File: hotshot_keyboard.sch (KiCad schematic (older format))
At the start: 25 parts, among them SW1 SW_Push, U1 ATmega32U4-AU, Y1 Crystal_GND24_Small

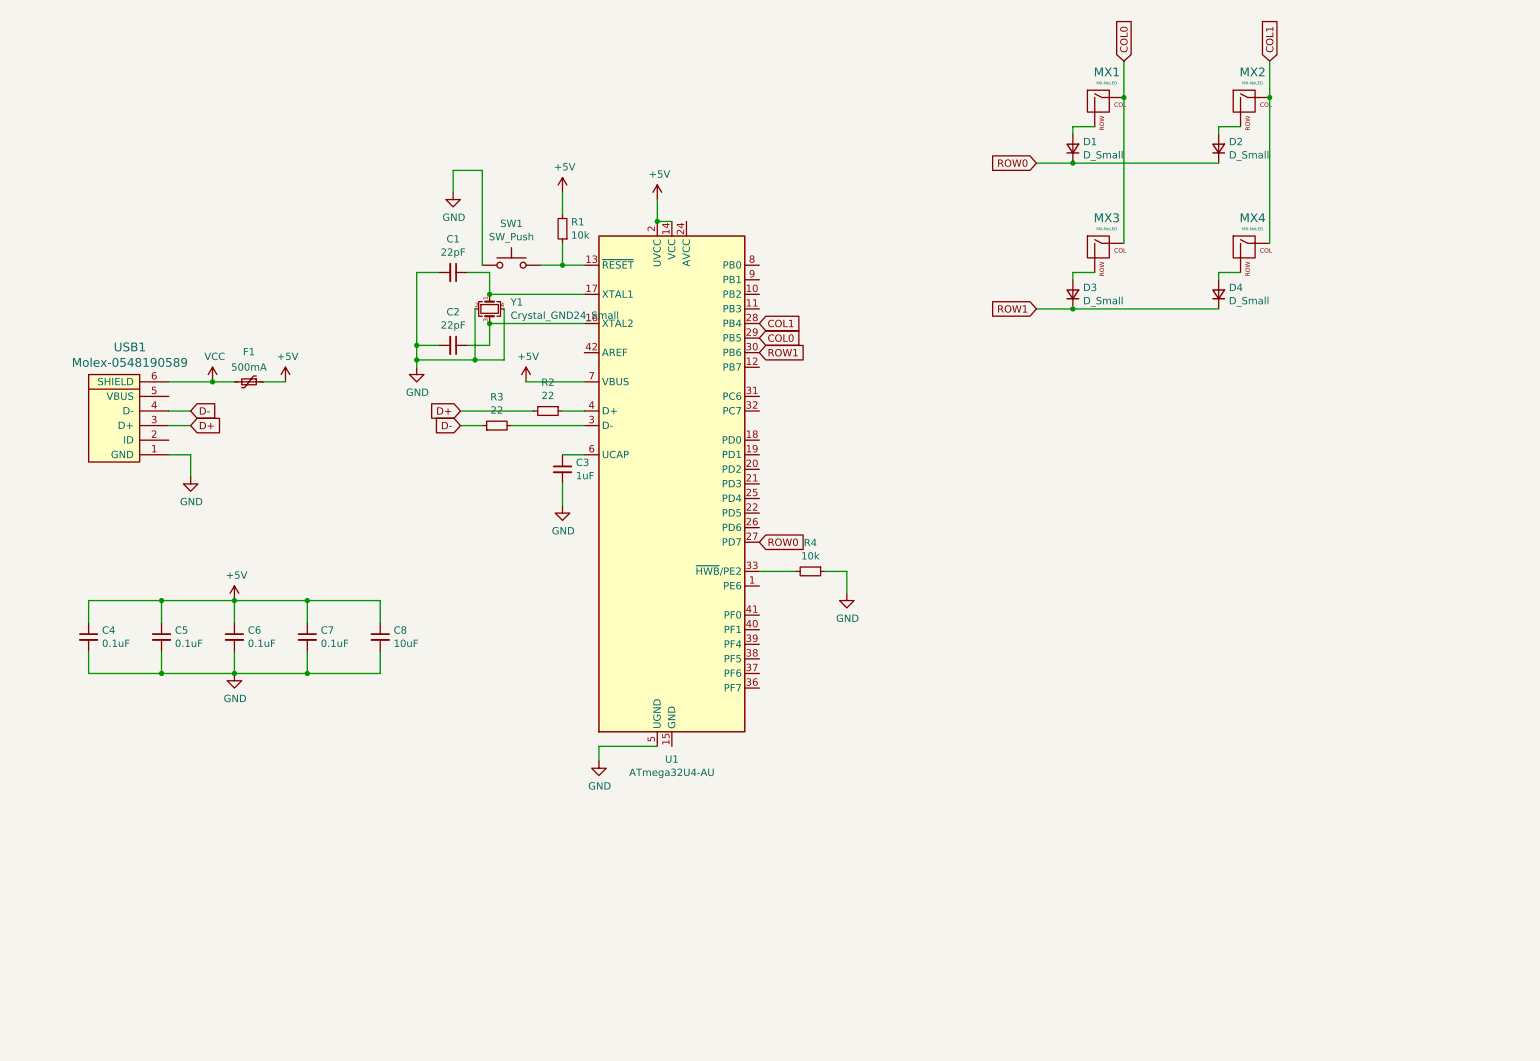
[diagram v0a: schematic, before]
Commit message: update schematics
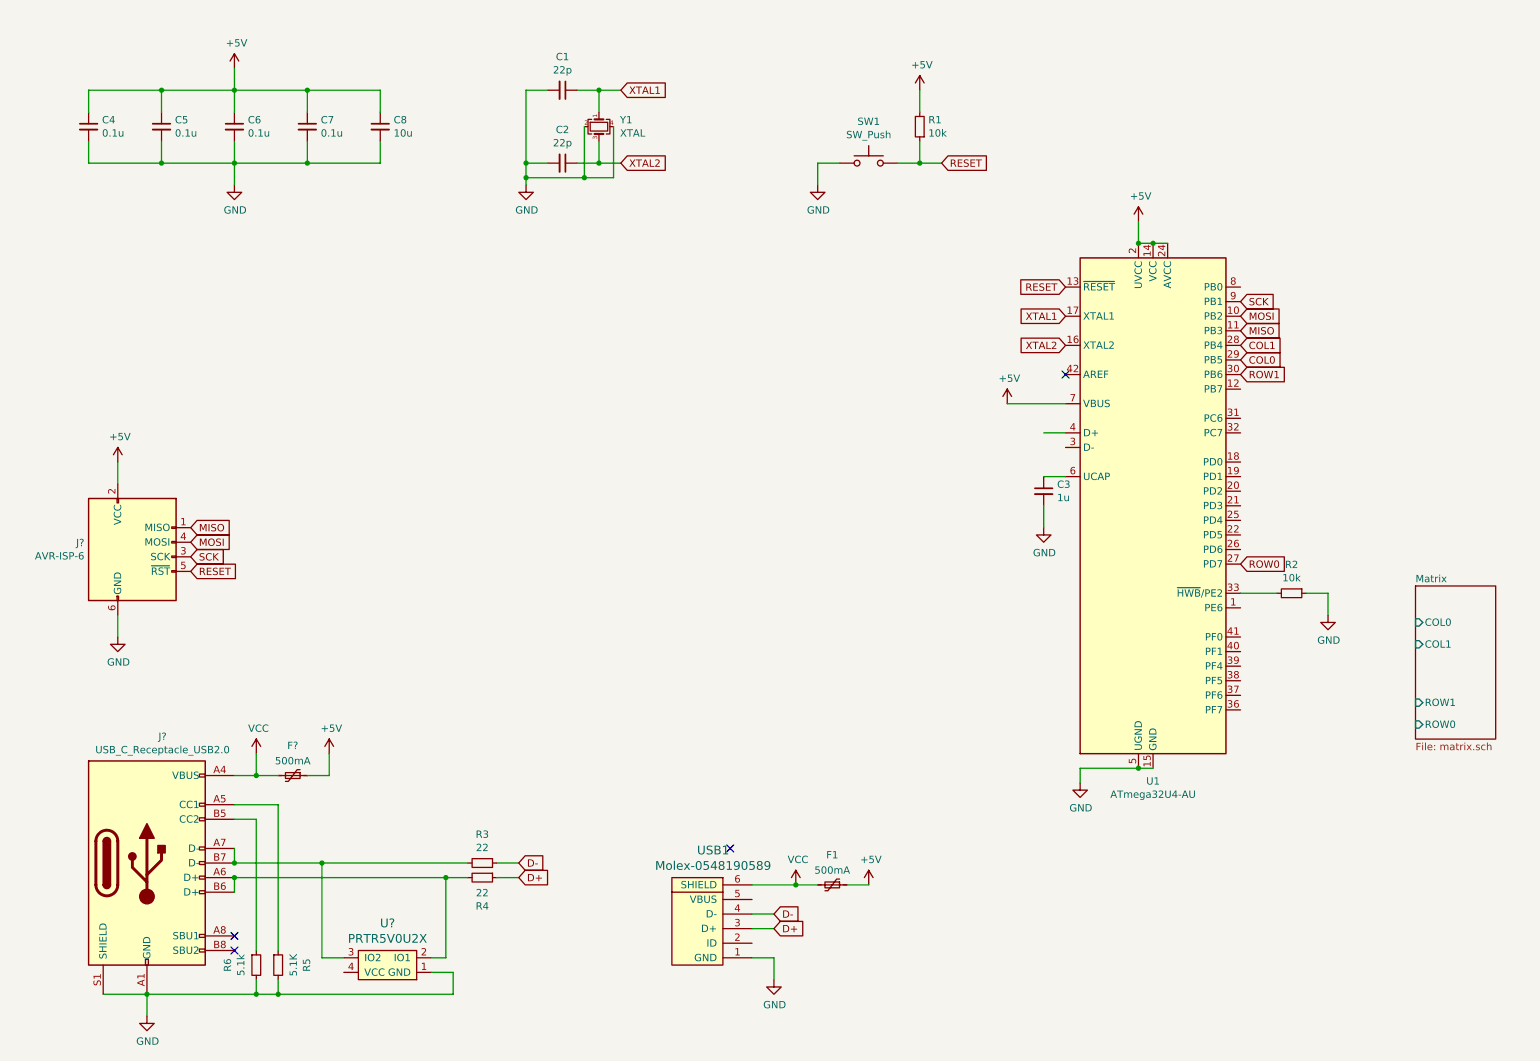
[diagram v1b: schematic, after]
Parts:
- removed D1, D2, D3, D4: D_Small, Diode_SMD:D_SOD-123, symbol Device:D_Small
- removed MX1, MX2, MX3, MX4: MX-NoLED, MX_Alps_Hybrid:MX-1U, symbol MX_Alps_Hybrid:MX-NoLED
- added F?: 500mA, Fuse:Fuse_1206_3216Metric, symbol Device:Polyfuse_Small
- added J?: AVR-ISP-6, symbol Connector:AVR-ISP-6
- added J?: USB_C_Receptacle_USB2.0, symbol Connector:USB_C_Receptacle_USB2.0
- added R5: 5.1K, Resistor_SMD:R_0805_2012Metric, symbol Device:R_Small
- added R6: 5.1k, Resistor_SMD:R_0805_2012Metric, symbol Device:R_Small
- added U?: PRTR5V0U2X, symbol random-keyboard-parts:PRTR5V0U2X
- C1, C2: value 22pF -> 22p
- C3: value 1uF -> 1u
- C4, C5, C6, C7: value 0.1uF -> 0.1u
- C8: value 10uF -> 10u
- Y1: value Crystal_GND24_Small -> XTAL
- renumbered R4 to R2, R2 to R3, R3 to R4
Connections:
- net +5V: now also U1.24 (AVCC), U1.44 (AVCC), F?.1, J?.2 (VCC)
- net D+: now also R4.1; no longer R3.2
- net D-: now also R3.1; no longer R4.1
- net GND: now also U1.15 (GND), U1.23 (GND), U1.35 (GND), U1.43 (GND), J?.6 (GND), J?.A1 (GND), J?.A12 (GND), J?.B1 (GND), J?.B12 (GND), J?.S1 (SHIELD), R5.2, R6.2, U?.1 (GND)
- net VCC: now also F?.2, J?.A4 (VBUS), J?.A9 (VBUS), J?.B4 (VBUS), J?.B9 (VBUS)
- net at U1.4 (D+): no longer R3.1
- net at R4.2: now also J?.A6 (D+), J?.B6 (D+), U?.2 (IO1); no longer U1.3 (D-)
- net XTAL1: now reaches C1.1, U1.17 (XTAL1), Y1.1
- net XTAL2: now reaches C2.1, U1.16 (XTAL2), Y1.3
- net RESET: now reaches R1.1, SW1.2, U1.13 (~RESET)
- net RESET: now also J?.5 (~RST)
- net MOSI: now reaches U1.10 (PB2)
- net MOSI: now also J?.4 (MOSI)
- net MISO: now reaches U1.11 (PB3)
- net MISO: now also J?.1 (MISO)
- net SCK: now reaches U1.9 (PB1)
- net SCK: now also J?.3 (SCK)
- new net: J?.A7 (D-), J?.B7 (D-), R3.2, U?.3 (IO2)
- new net: J?.A5 (CC1), R5.1
- new net: J?.B5 (CC2), R6.1
- no-connect marks 0 -> 4
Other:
- moved on the sheet: C1, C2, C3, C4, C5, C6, C7, C8, F1, R1, R2, R3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

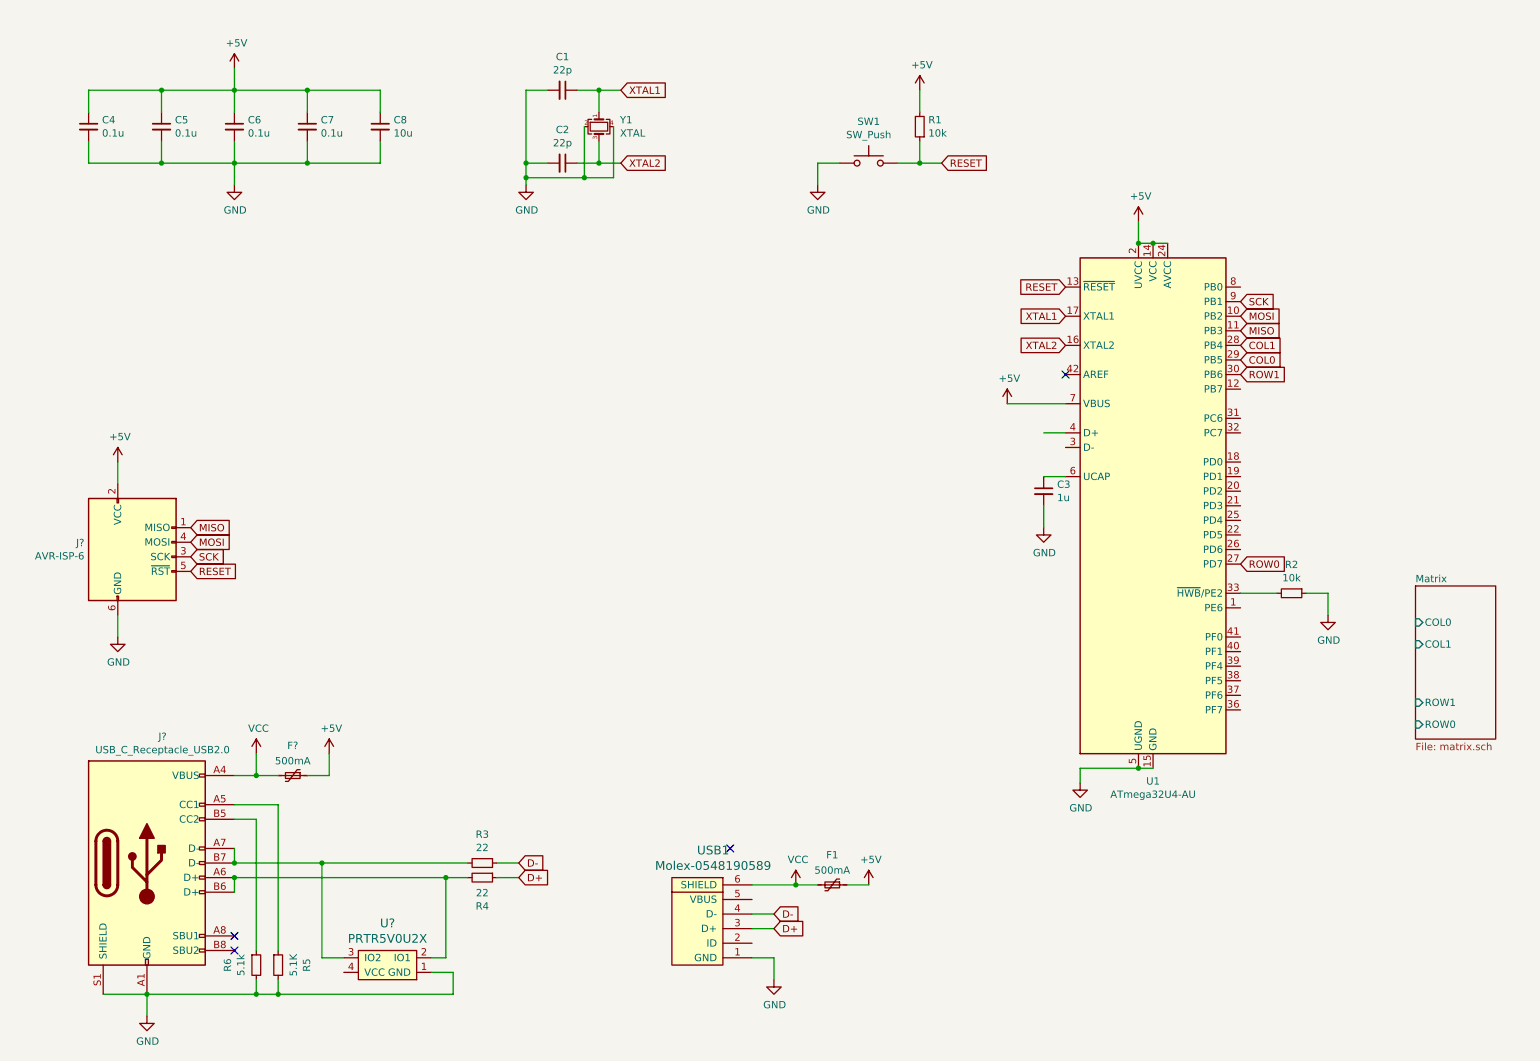
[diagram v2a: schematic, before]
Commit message: update schematics
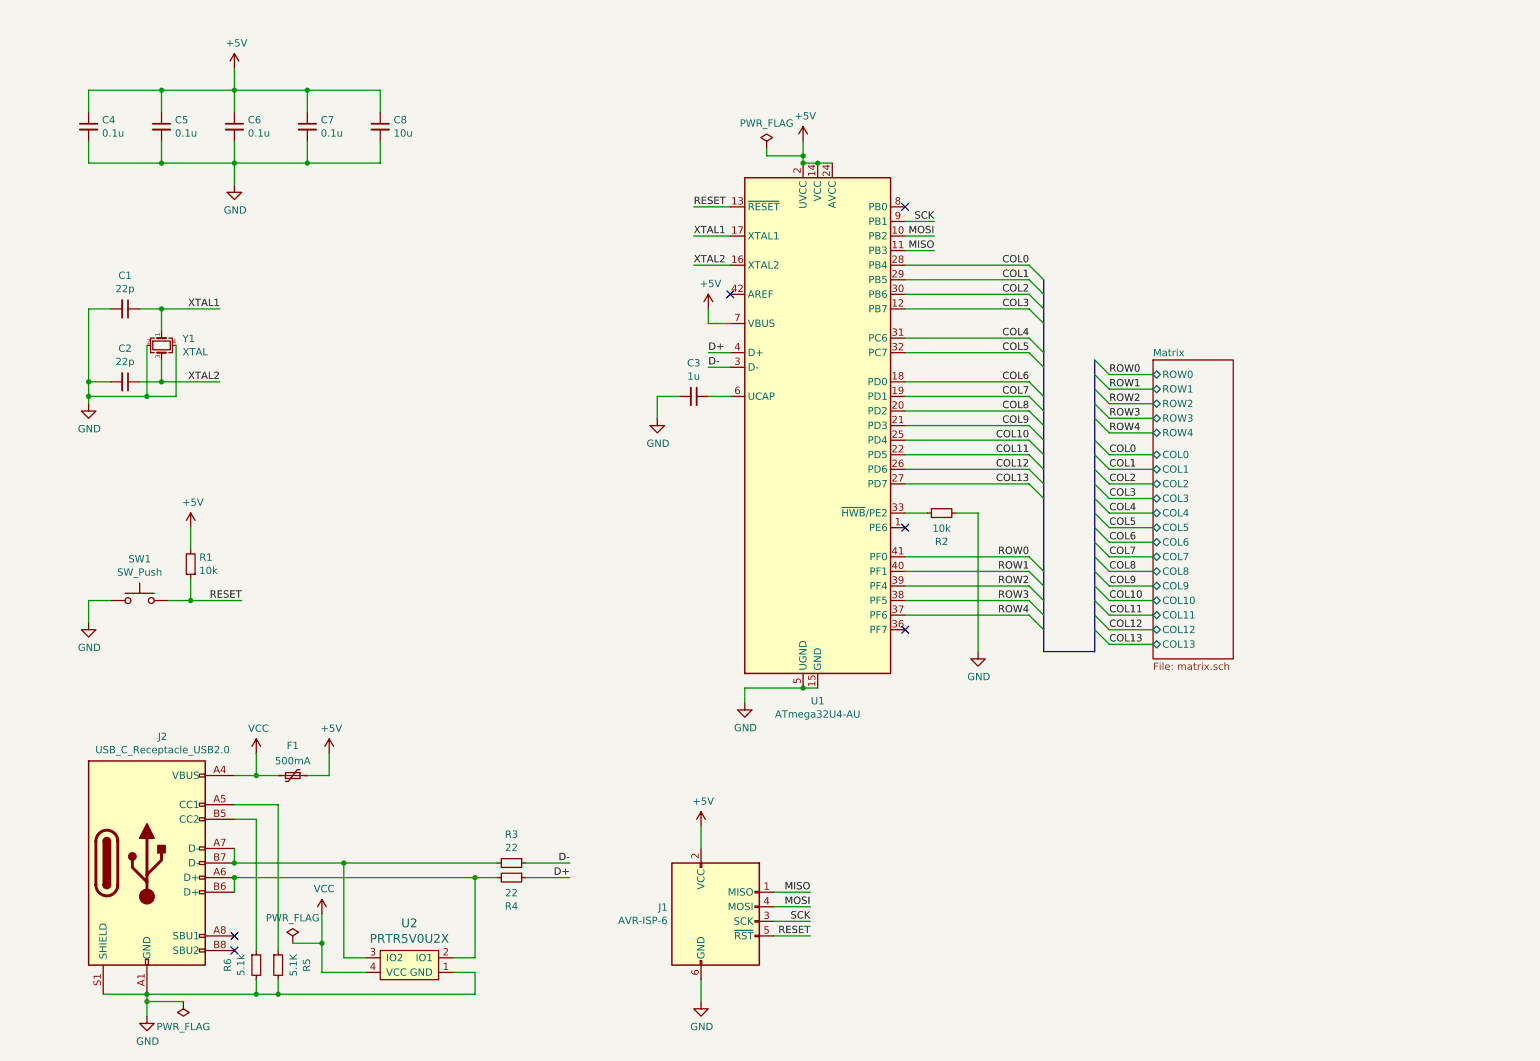
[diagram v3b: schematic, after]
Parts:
- removed F1: 500mA, Fuse:Fuse_1206_3216Metric, symbol Device:Polyfuse_Small
- removed USB1: Molex-0548190589, random-keyboard-parts:Molex-0548190589, symbol random-keyboard-parts:Molex-0548190589
- gave numbers to parts that had none: 4
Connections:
- net COL0: now also U1.28 (PB4); no longer U1.29 (PB5)
- net COL1: now also U1.29 (PB5); no longer U1.28 (PB4)
- net D+: now also U1.4 (D+)
- net D-: now also U1.3 (D-)
- net GND: now also R2.2; no longer R2.1
- net ROW0: now also U1.41 (PF0); no longer U1.27 (PD7)
- net ROW1: now also U1.40 (PF1); no longer U1.30 (PB6)
- net VCC: now also U2.4 (VCC)
- net at U1.33 (~HWB~/PE2): now also R2.1; no longer R2.2
- net COL3: now reaches U1.12 (PB7)
- net COL6: now reaches U1.18 (PD0)
- net COL7: now reaches U1.19 (PD1)
- net COL8: now reaches U1.20 (PD2)
- net COL9: now reaches U1.21 (PD3)
- net COL11: now reaches U1.22 (PD5)
- net COL10: now reaches U1.25 (PD4)
- net COL12: now reaches U1.26 (PD6)
- net COL4: now reaches U1.31 (PC6)
- net COL5: now reaches U1.32 (PC7)
- net ROW4: now reaches U1.37 (PF6)
- net ROW3: now reaches U1.38 (PF5)
- net ROW2: now reaches U1.39 (PF4)
- new net COL13: U1.27 (PD7)
- new net COL2: U1.30 (PB6)
- no-connect marks 4 -> 6
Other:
- moved on the sheet: C1, C2, J1, R1, R2, R3, R4, SW1, U1, U2, Y1

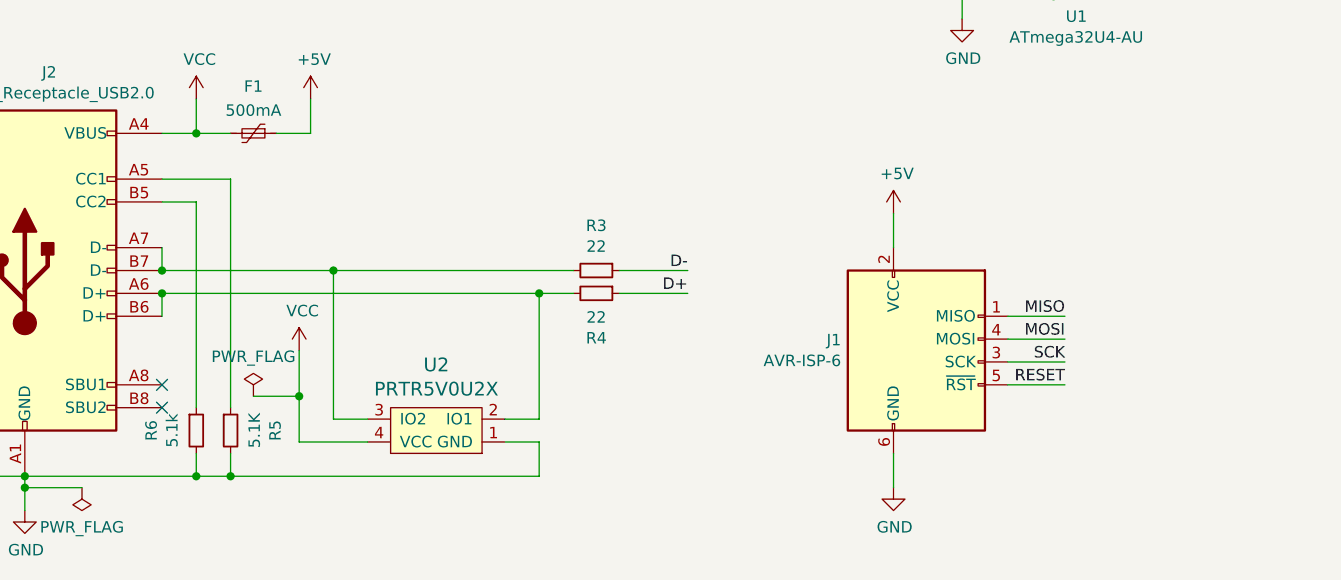
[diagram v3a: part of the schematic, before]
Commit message: update pcb
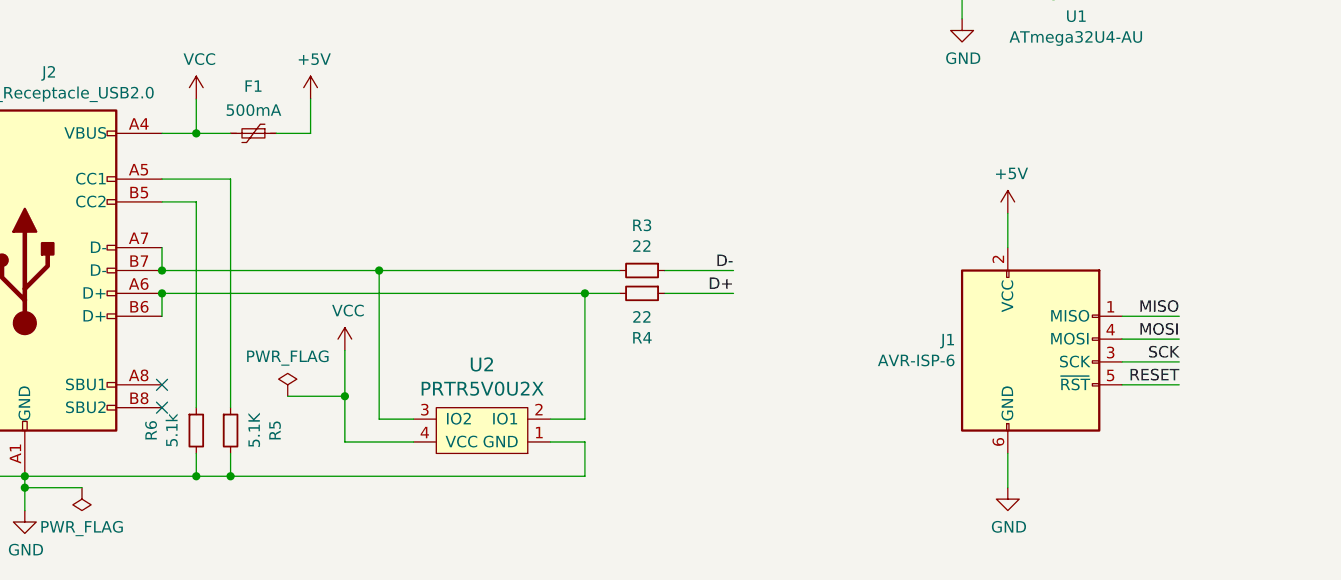
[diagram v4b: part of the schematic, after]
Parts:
- C1, C2, C3, C4, C5, C6, C7, C8: footprint Capacitor_SMD:C_0805_2012Metric -> Capacitor_SMD:C_0805_2012Metric_Pad1.18x1.45mm_HandSolder
- F1: footprint Fuse:Fuse_1206_3216Metric -> Fuse:Fuse_1206_3216Metric_Pad1.42x1.75mm_HandSolder
- J1: footprint (none) -> random-keyboard-parts:Reset_Pretty-Mask
- J2: footprint (none) -> Connector_USB:USB_C_Receptacle_HRO_TYPE-C-31-M-12
- R1, R2, R3, R4, R5, R6: footprint Resistor_SMD:R_0805_2012Metric -> Resistor_SMD:R_0805_2012Metric_Pad1.20x1.40mm_HandSolder
- SW1: footprint random-keyboard-parts:SKQG-1155865 -> Button_Switch_SMD:SW_SPST_SKQG_WithStem
- U2: footprint (none) -> random-keyboard-parts:SOT143B
- Y1: footprint Crystal:Crystal_SMD_3225-4Pin_3.2x2.5mm -> Crystal:Crystal_SMD_3225-4Pin_3.2x2.5mm_HandSoldering
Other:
- moved on the sheet: J1, R3, R4, U2
